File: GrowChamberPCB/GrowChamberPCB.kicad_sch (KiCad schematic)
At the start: 28 parts, among them J1 Screw_Terminal_01x02, J2 Conn_01x03_Pin, J4 Conn_01x02_Socket, U2 MCP1826S, U4 TC4428xOA, U5 W25Q128JVS

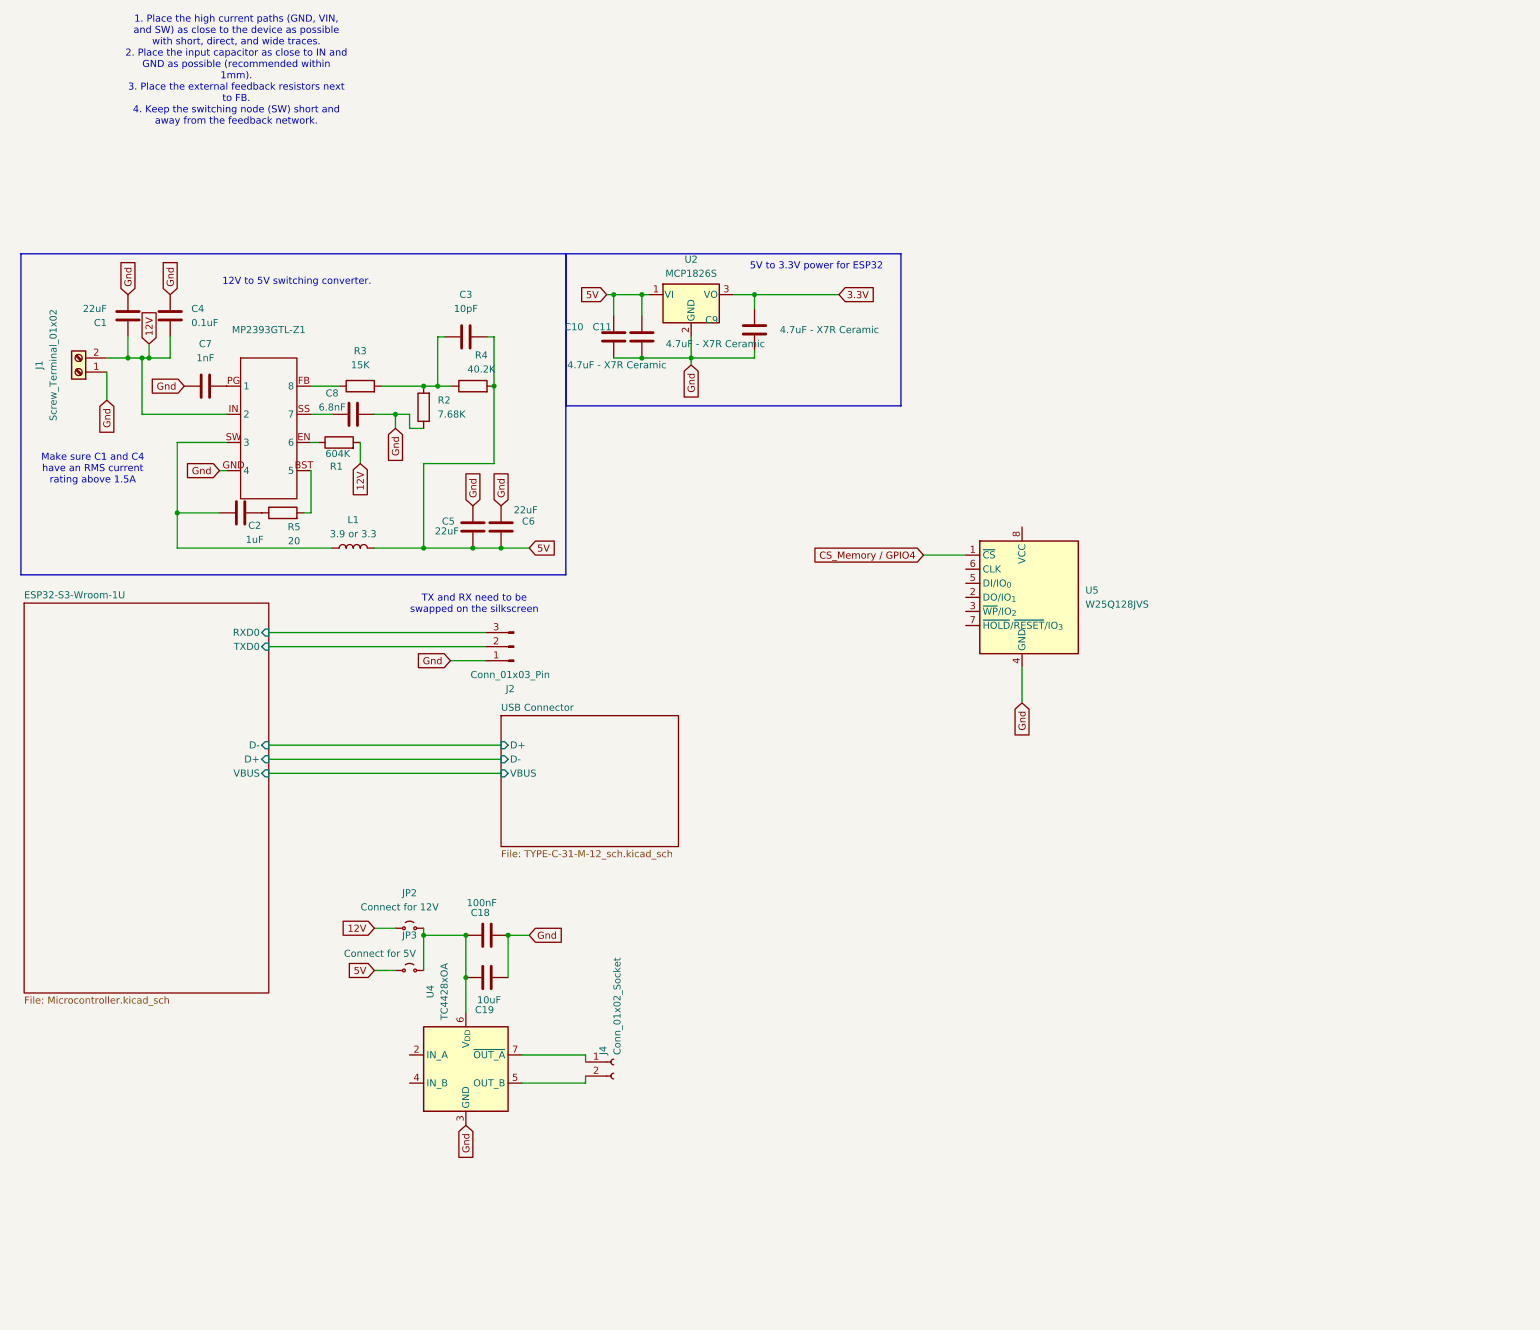
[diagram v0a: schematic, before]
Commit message: bunch o stuff
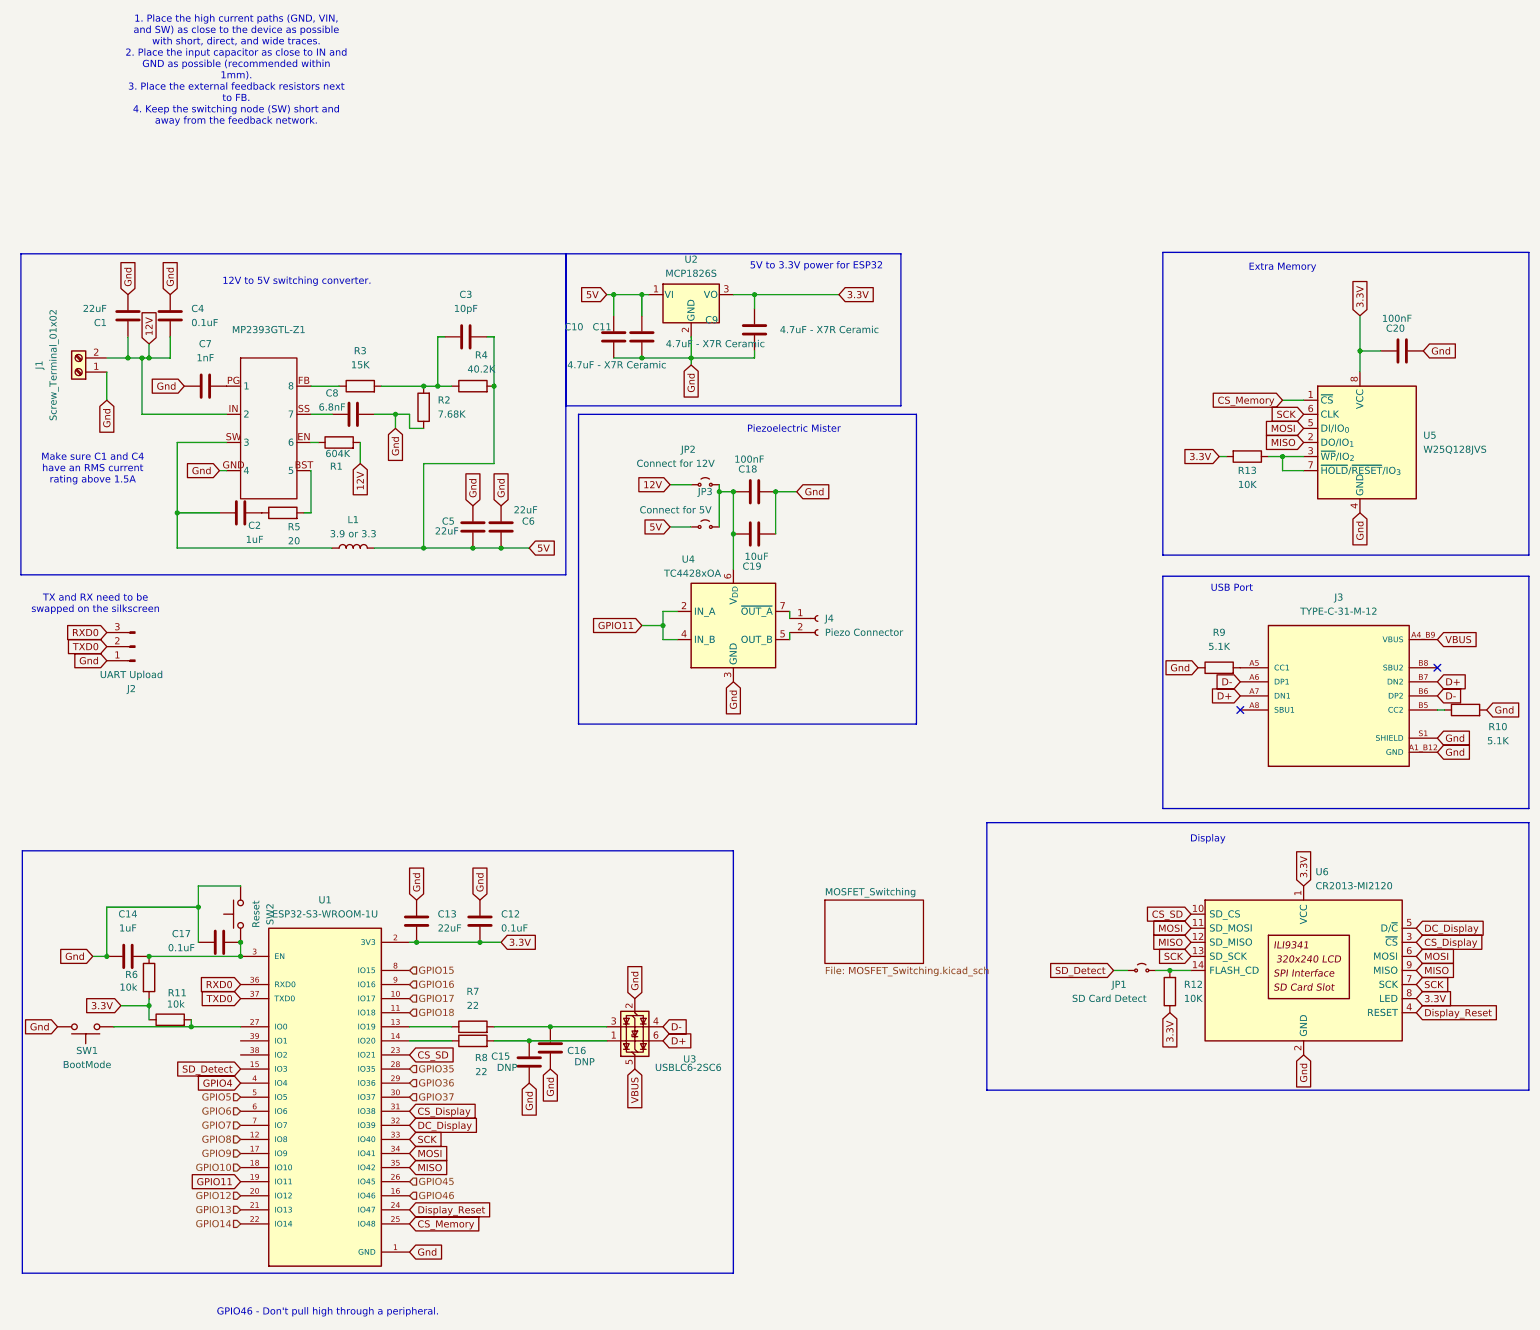
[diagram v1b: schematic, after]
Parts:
- added C12, C17: 0.1uF, symbol Device:C
- added C13: 22uF, symbol Device:C
- added C14: 1uF, symbol Device:C
- added C15, C16: DNP, symbol Device:C
- added C20: 100nF, symbol Device:C
- added J3: TYPE-C-31-M-12, Connector_USB:USB_C_Receptacle_HRO_TYPE-C-31-M-12, symbol Custom_Library:TYPE-C-31-M-12
- added JP1: SD Card Detect, symbol Jumper:Jumper_2_Small_Open
- added R10, R9: 5.1K, symbol Device:R
- added R11, R6: 10k, symbol Device:R
- added R12, R13: 10K, symbol Device:R
- added R7, R8: 22, symbol Device:R
- added SW1: BootMode, symbol Switch:SW_Push
- added SW2: Reset, symbol Switch:SW_Push
- added U1: ESP32-S3-WROOM-1U, ESP32-S3-WROOM-1U:XCVR_ESP32-S3-WROOM-1U, symbol Custom_Library:ESP32-S3-WROOM-1U
- added U3: USBLC6-2SC6, Package_TO_SOT_SMD:SOT-23-6, symbol Power_Protection:USBLC6-2SC6
- added U6: CR2013-MI2120, Display:CR2013-MI2120, symbol Driver_Display:CR2013-MI2120
- J2: value Conn_01x03_Pin -> UART Upload
- J4: value Conn_01x02_Socket -> Piezo Connector
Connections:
- net 3.3V: now also U5.8 (VCC), C12.2, C13.2, C20.2, R11.1, R12.1, R13.2, R6.2, U1.2 (3V3), U6.1 (VCC), U6.8 (LED)
- net GPIO11: now reaches U4.2 (IN_A)
- net GPIO11: now also U4.4 (IN_B), U1.19 (IO11)
- net MISO: now reaches U5.2 (DO/IO_{1})
- net MISO: now also U1.35 (IO42), U6.12 (SD_MISO), U6.9 (MISO)
- net at U5.3 (~{WP}/IO_{2}): now also U5.7 (~{HOLD}/~{RESET}/IO_{3}), R13.1
- net MOSI: now reaches U5.5 (DI/IO_{0})
- net MOSI: now also U1.34 (IO41), U6.11 (SD_MOSI), U6.6 (MOSI)
- net SCK: now reaches U5.6 (CLK)
- net SCK: now also U1.33 (IO40), U6.13 (SD_SCK), U6.7 (SCK)
- net CS_Memory / GPIO4 renamed CS_Memory
- net CS_Memory: now also U1.25 (IO48)
- net ESP32-S3-Wroom-1U/RXD0 renamed RXD0
- net RXD0: now also U1.36 (RXD0)
- net ESP32-S3-Wroom-1U/TXD0 renamed TXD0
- net TXD0: now also U1.37 (TXD0)
- net Gnd renamed GND
- net GND: now also C12.1, C13.1, C14.1, C15.2, C16.2, C17.1, C20.1, J3.A1_B12 (GND), J3.B1_A12 (GND), J3.S1 (SHIELD), J3.S2 (SHIELD), J3.S3 (SHIELD), J3.S4 (SHIELD), R10.2, R9.1, SW1.2, SW2.2, U1.1 (GND), U1.40 (GND), U1.41_1 (GND), U1.41_2 (GND), U1.41_3 (GND), U1.41_4 (GND), U1.41_5 (GND), U1.41_6 (GND), U1.41_7 (GND), U1.41_8 (GND), U1.41_9 (GND), U3.2 (GND), U6.2 (GND)
- new net: R7.1, U1.13 (IO19)
- new net: R8.1, U1.14 (IO20)
- new net: R11.2, SW1.1, U1.27 (IO0)
- new net: C14.2, C17.2, R6.1, SW2.1, U1.3 (EN)
- new net: JP1.2 (B), R12.2, U6.14 (FLASH_CD)
- new net: C15.1, R8.2, U3.1 (I/O1)
- new net: J3.A5 (CC1), R9.2
- new net: J3.B5 (CC2), R10.1
- new net: C16.1, R7.2, U3.3 (I/O2)
- new net CS_Display: U1.31 (IO38), U6.3 (~{CS})
- new net CS_SD: U1.23 (IO21), U6.10 (SD_CS)
- new net D+: J3.A7 (DN1), J3.B7 (DN2), U3.6 (I/O1)
- new net D-: J3.A6 (DP1), J3.B6 (DP2), U3.4 (I/O2)
- new net DC_Display: U1.32 (IO39), U6.5 (D/~{C})
- new net Display_Reset: U1.24 (IO47), U6.4 (RESET)
- new net GPIO10: U1.18 (IO10)
- new net GPIO12: U1.20 (IO12)
- new net GPIO13: U1.21 (IO13)
- new net GPIO14: U1.22 (IO14)
- new net GPIO15: U1.8 (IO15)
- new net GPIO16: U1.9 (IO16)
- new net GPIO17: U1.10 (IO17)
- new net GPIO18: U1.11 (IO18)
- new net GPIO35: U1.28 (IO35)
- new net GPIO36: U1.29 (IO36)
- new net GPIO37: U1.30 (IO37)
- new net GPIO4: U1.4 (IO4)
- new net GPIO45: U1.26 (IO45)
- new net GPIO46: U1.16 (IO46)
- new net GPIO5: U1.5 (IO5)
- new net GPIO6: U1.6 (IO6)
- new net GPIO7: U1.7 (IO7)
- new net GPIO8: U1.12 (IO8)
- new net GPIO9: U1.17 (IO9)
- new net SD_Detect: JP1.1 (A), U1.15 (IO3)
- new net VBUS: J3.A4_B9 (VBUS), J3.B4_A9 (VBUS), U3.5 (VBUS)
- no-connect marks 0 -> 2
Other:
- removed sheet ESP32-S3-Wroom-1U
- removed sheet USB Connector
- added sheet MOSFET_Switching (MOSFET_Switching.kicad_sch)
- note added: "Display"
- note added: "Extra Memory"
- note added: "GPIO46 - Don't pull high through a peripheral."
- note added: "Piezoelectric Mister"
- note added: "USB Port"
- moved on the sheet: C18, C19, J2, J4, JP2, JP3, U4, U5
